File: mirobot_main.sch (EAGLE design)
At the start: 26 parts, among them IC1 ULN2003AN, IC2 ULN2003AN, IC3 ATMEGA 328, IC4 5V, IC5 3.3V, Q2 16M, X1 22-23-2051, X2 22-23-2051

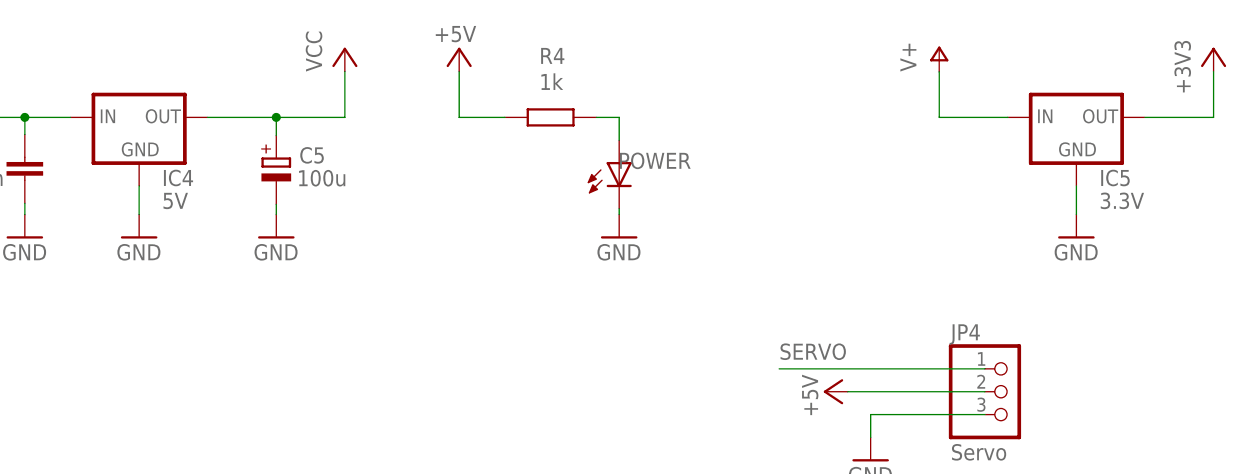
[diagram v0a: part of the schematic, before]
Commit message: Version 1.2 of the Mirobot PCB
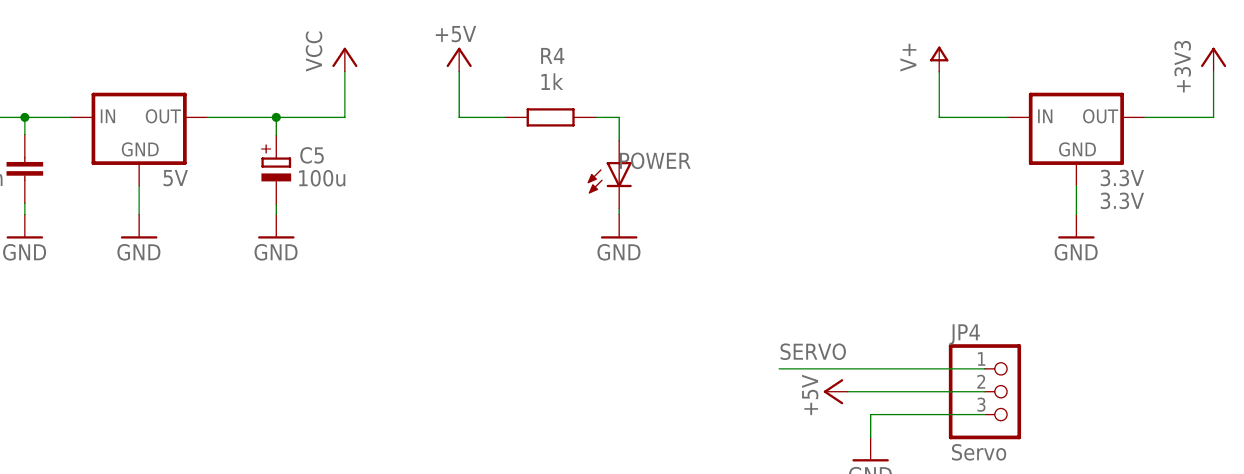
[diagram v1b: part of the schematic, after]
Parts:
- removed IC4: 5V, v-reg:78LXX
- added 5V: (no value), v-reg:78MXXS
- renumbered IC5 to 3.3V
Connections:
- net GND: now also 5V.GND; no longer IC4.GND
- net V+: now also 5V.IN; no longer IC4.IN
- net VCC: now also 5V.OUT; no longer IC4.OUT
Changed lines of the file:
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@@
 <part name="POWER" library="led" deviceset="LED" device="3MM"/>
 <part name="GND19" library="supply1" deviceset="GND" device=""/>
-<part name="IC4" library="v-reg" deviceset="78LXX" device="" value="5V"/>
 <part name="C4" library="rcl" deviceset="C-EU" device="050-025X075" value="100n"/>
 <part name="GND8" library="supply1" deviceset="GND" device=""/>
@@
 <part name="R2" library="rcl" deviceset="R-EU_" device="0204/5" value="1k"/>
 <part name="GND3" library="supply1" deviceset="GND" device=""/>
-<part name="IC5" library="v-reg" deviceset="78LXX" device="" value="3.3V"/>
+<part name="3.3V" library="v-reg" deviceset="78LXX" device="" value="3.3V"/>
 <part name="P+11" library="supply1" deviceset="V+" device=""/>
 <part name="GND14" library="supply1" deviceset="GND" device=""/>
@@
 <part name="X2" library="con-molex" deviceset="22-23-2051" device=""/>
 <part name="P+8" library="supply1" deviceset="+5V" device=""/>
+<part name="5V" library="v-reg" deviceset="78MXXS" device=""/>
 </parts>
 <sheets>
@@
 </instance>
 <instance part="GND19" gate="1" x="-91.44" y="65.405"/>
-<instance part="IC4" gate="1" x="-30.48" y="81.28"/>
 <instance part="C4" gate="G$1" x="-99.06" y="34.671" smashed="yes" rot="R180">
 <attribute name="NAME" x="-100.584" y="34.29" size="1.778" layer="95" rot="R180"/>
@@
 <instance part="R2" gate="G$1" x="-5.08" y="-53.34" rot="R90"/>
 <instance part="GND3" gate="1" x="-5.08" y="-63.5"/>
-<instance part="IC5" gate="1" x="73.66" y="81.28"/>
+<instance part="3.3V" gate="1" x="73.66" y="81.28"/>
 <instance part="P+11" gate="1" x="58.42" y="88.9"/>
 <instance part="GND14" gate="1" x="73.66" y="67.945"/>
@@
 <attribute name="VALUE" x="6.985" y="91.44" size="1.778" layer="96" rot="R180"/>
 </instance>
+<instance part="5V" gate="A" x="-30.48" y="81.28"/>
 </instances>
 <busses>
@@
 <wire x1="-30.48" y1="73.66" x2="-30.48" y2="70.485" width="0.1524" layer="91"/>
 <pinref part="GND6" gate="1" pin="GND"/>
-<pinref part="IC4" gate="1" pin="GND"/>
+<pinref part="5V" gate="A" pin="GND"/>
 </segment>
 <segment>
@@
 </segment>
 <segment>
-<pinref part="IC5" gate="1" pin="GND"/>
+<pinref part="3.3V" gate="1" pin="GND"/>
 <wire x1="73.66" y1="73.66" x2="73.66" y2="70.485" width="0.1524" layer="91"/>
 <pinref part="GND14" gate="1" pin="GND"/>
@@
 <junction x="-15.24" y="81.28"/>
 <pinref part="C5" gate="G$1" pin="+"/>
-<pinref part="IC4" gate="1" pin="OUT"/>
 <pinref part="P+5" gate="VCC" pin="VCC"/>
+<pinref part="5V" gate="A" pin="OUT"/>
 </segment>
 <segment>
@@
 <junction x="-55.88" y="81.28"/>
 <pinref part="C8" gate="G$1" pin="+"/>
-<pinref part="IC4" gate="1" pin="IN"/>
 <pinref part="C7" gate="G$1" pin="2"/>
 <wire x1="-43.18" y1="79.375" x2="-43.18" y2="81.28" width="0.1524" layer="91"/>
 <junction x="-43.18" y="81.28"/>
 <wire x1="-71.12" y1="81.28" x2="-55.88" y2="81.28" width="0.1524" layer="91"/>
+<pinref part="5V" gate="A" pin="IN"/>
 </segment>
 <segment>
@@
 <segment>
 <pinref part="P+11" gate="1" pin="V+"/>
-<pinref part="IC5" gate="1" pin="IN"/>
+<pinref part="3.3V" gate="1" pin="IN"/>
 <wire x1="58.42" y1="86.36" x2="58.42" y2="81.28" width="0.1524" layer="91"/>
 <wire x1="58.42" y1="81.28" x2="66.04" y2="81.28" width="0.1524" layer="91"/>
@@
 <net name="+3V3" class="0">
 <segment>
-<pinref part="IC5" gate="1" pin="OUT"/>
+<pinref part="3.3V" gate="1" pin="OUT"/>
 <wire x1="81.28" y1="81.28" x2="88.9" y2="81.28" width="0.1524" layer="91"/>
 <wire x1="88.9" y1="81.28" x2="88.9" y2="86.36" width="0.1524" layer="91"/>

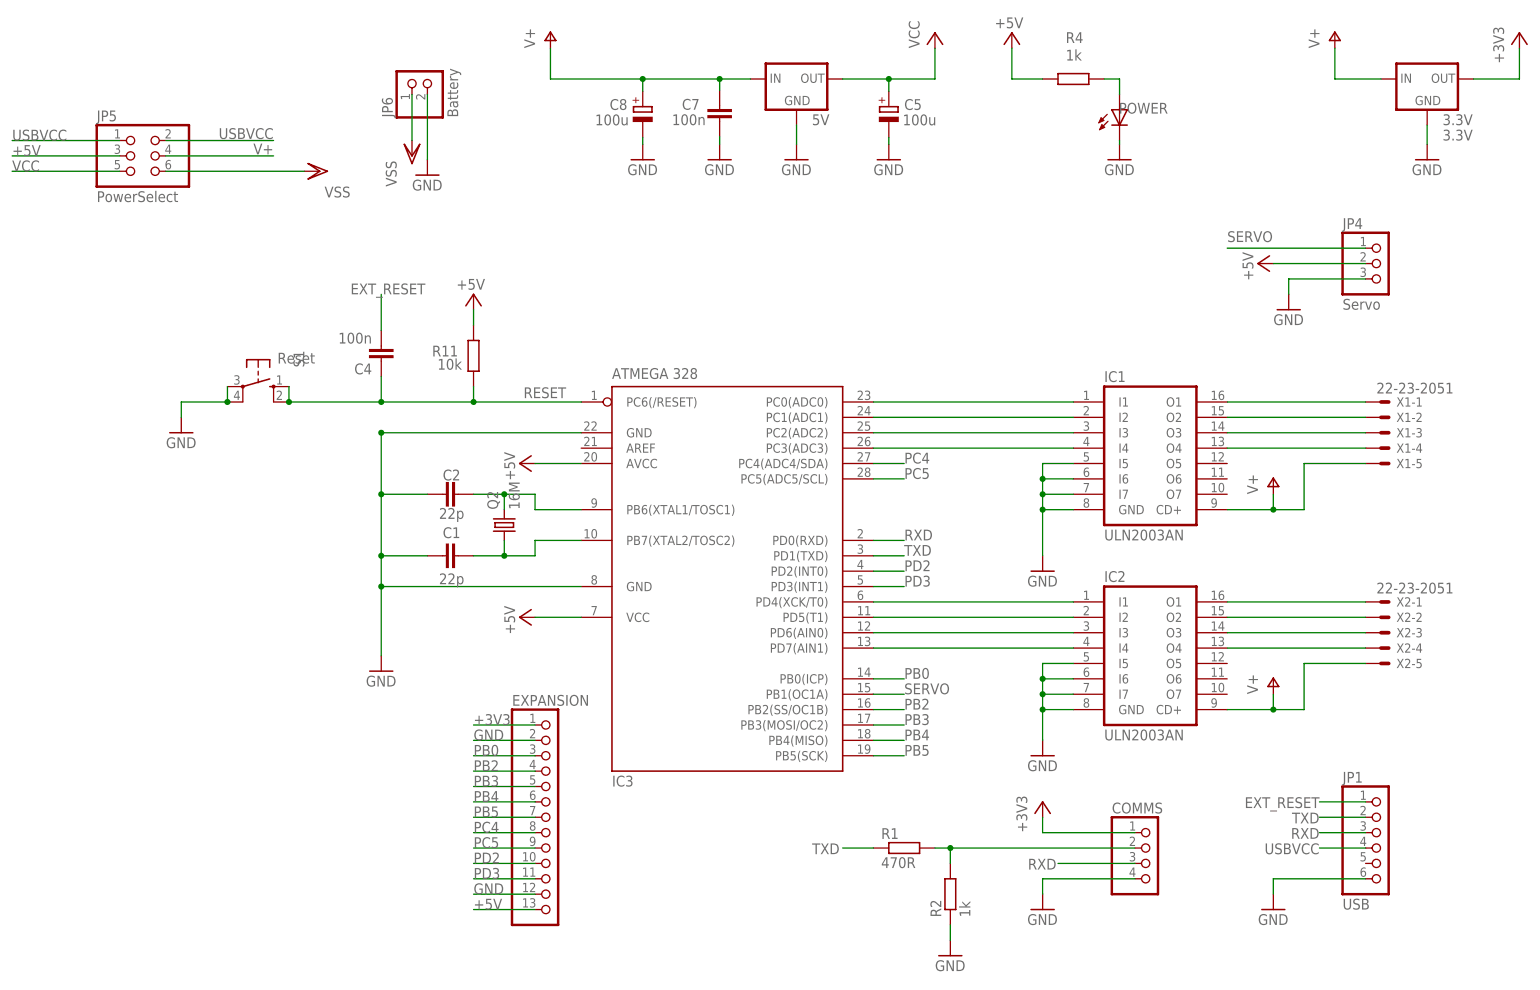
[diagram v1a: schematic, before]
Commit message: Version 1.3 of the Mirobot PCB
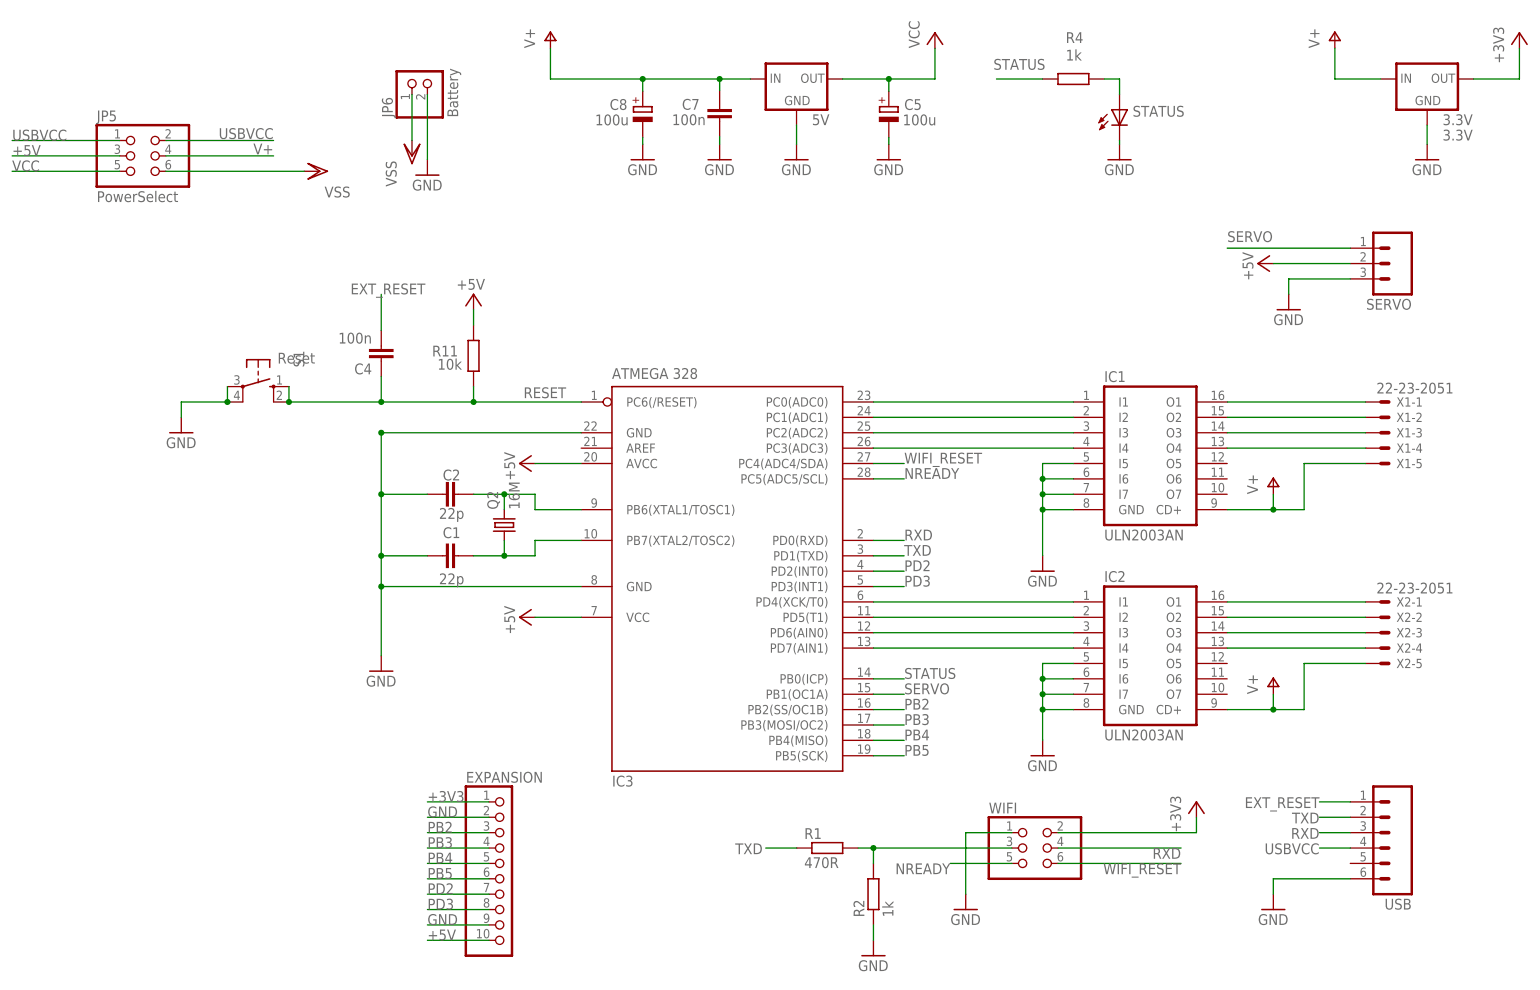
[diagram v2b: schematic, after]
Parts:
- removed COMMS: (no value), pinhead:PINHD-1X4
- removed JP1: USB, pinhead:PINHD-1X6
- removed JP4: Servo, pinhead:PINHD-1X3
- removed POWER: (no value), led:LED3MM
- added SERVO: (no value), SparkFun-Connectors:M03LOCK_LONGPADS
- added STATUS: (no value), Child-Friendly-Parts:LED3MM
- added USB: (no value), SparkFun-Connectors:M06LOCK_LONGPADS
- added WIFI: (no value), Child-Friendly-Parts:PINHD-2X3
- 3.3V: device v-reg:78LXX -> Child-Friendly-Parts:78LXX
- C1, C2: device rcl:C-EU025-024X044 -> Child-Friendly-Parts:C-EU025-024X044
- C4, C7: device rcl:C-EU050-025X075 -> Child-Friendly-Parts:C-EU050-025X075
- C5, C8: device rcl:CPOL-EUE2-5 -> Child-Friendly-Parts:CPOL-EUE2-5
- EXPANSION: device pinhead:PINHD-1X13 -> pinhead:PINHD-1X10
- JP5: device pinhead:PINHD-2X3 -> Child-Friendly-Parts:PINHD-2X3
- Q2: device crystal:CRYSTALHC49S -> Child-Friendly-Parts:CRYSTALHC49S
- R1, R11, R2, R4: device rcl:R-EU_0204/5 -> Child-Friendly-Parts:R-EU_0204/5
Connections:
- removed net PB0: EXPANSION.3, IC3.PB0(ICP)
- removed net PC4: EXPANSION.8, IC3.PC4(ADC4/SDA)
- removed net PC5: EXPANSION.9, IC3.PC5(ADC5/SCL)
- new net NREADY: IC3.PC5(ADC5/SCL), WIFI.5
- new net STATUS: IC3.PB0(ICP), R4.2
- new net WIFI_RESET: IC3.PC4(ADC4/SDA), WIFI.6
- net +3V3: now also WIFI.2; no longer COMMS.1
- net +5V: now also EXPANSION.10, SERVO.2; no longer EXPANSION.13, JP4.2, R4.2
- net EXT_RESET: now also USB.1; no longer JP1.1
- net GND: now also EXPANSION.9, SERVO.3, STATUS.C, USB.6, WIFI.1; no longer COMMS.4, EXPANSION.12, JP1.6, JP4.3, POWER.C
- net N$19: now also WIFI.3; no longer COMMS.2
- net N$20: now also STATUS.A; no longer POWER.A
- net PB2: now also EXPANSION.3; no longer EXPANSION.4
- net PB3: now also EXPANSION.4; no longer EXPANSION.5
- net PB4: now also EXPANSION.5; no longer EXPANSION.6
- net PB5: now also EXPANSION.6; no longer EXPANSION.7
- net PD2: now also EXPANSION.7; no longer EXPANSION.10
- net PD3: now also EXPANSION.8; no longer EXPANSION.11
- net RXD: now also USB.3, WIFI.4; no longer COMMS.3, JP1.3
- net SERVO: now also SERVO.1; no longer JP4.1
- net TXD: now also USB.2; no longer JP1.2
- net USBVCC: now also USB.4; no longer JP1.4
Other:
- moved on the sheet: R1, R2

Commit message: Version 1.4 of the mian PCB and 1.1 of the WiFi PCB
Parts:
- JP6: device pinhead:PINHD-1X2 -> Child-Friendly-Parts:PINHD-1X2
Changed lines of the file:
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@@
 <part name="P+6" library="supply1" deviceset="V+" device=""/>
 <part name="P+7" library="supply1" deviceset="V+" device=""/>
-<part name="JP6" library="pinhead" deviceset="PINHD-1X2" device="" value="Battery"/>
+<part name="JP6" library="Child-Friendly-Parts" deviceset="PINHD-1X2" device="" value="Battery"/>
 <part name="P+9" library="supply1" deviceset="V+" device=""/>
 <part name="JP5" library="Child-Friendly-Parts" deviceset="PINHD-2X3" device="" value="PowerSelect"/>
